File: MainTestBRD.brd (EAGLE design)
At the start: 64.4 x 62.3 mm, 27 parts, among them IC1 LM3940IMP-3.3, U1 ATMEGA128-SMD

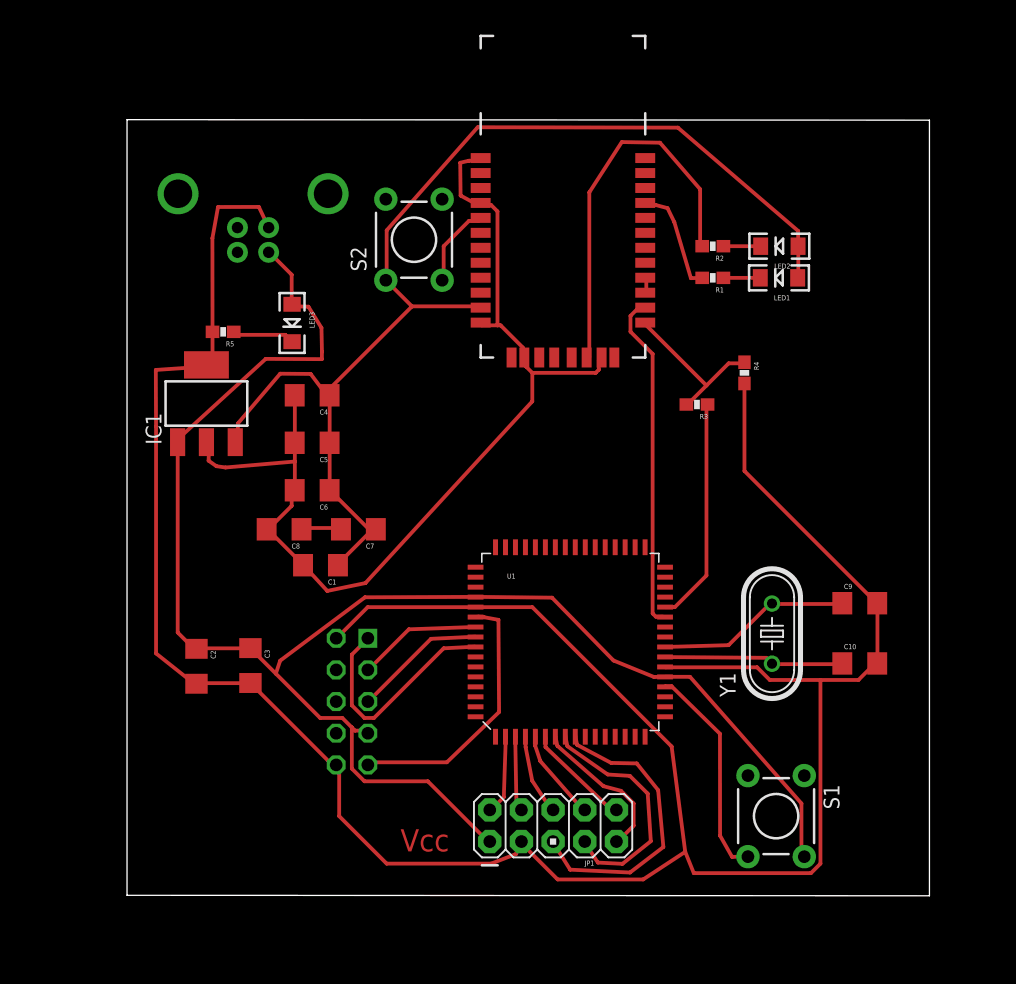
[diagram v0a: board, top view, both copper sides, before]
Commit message: __
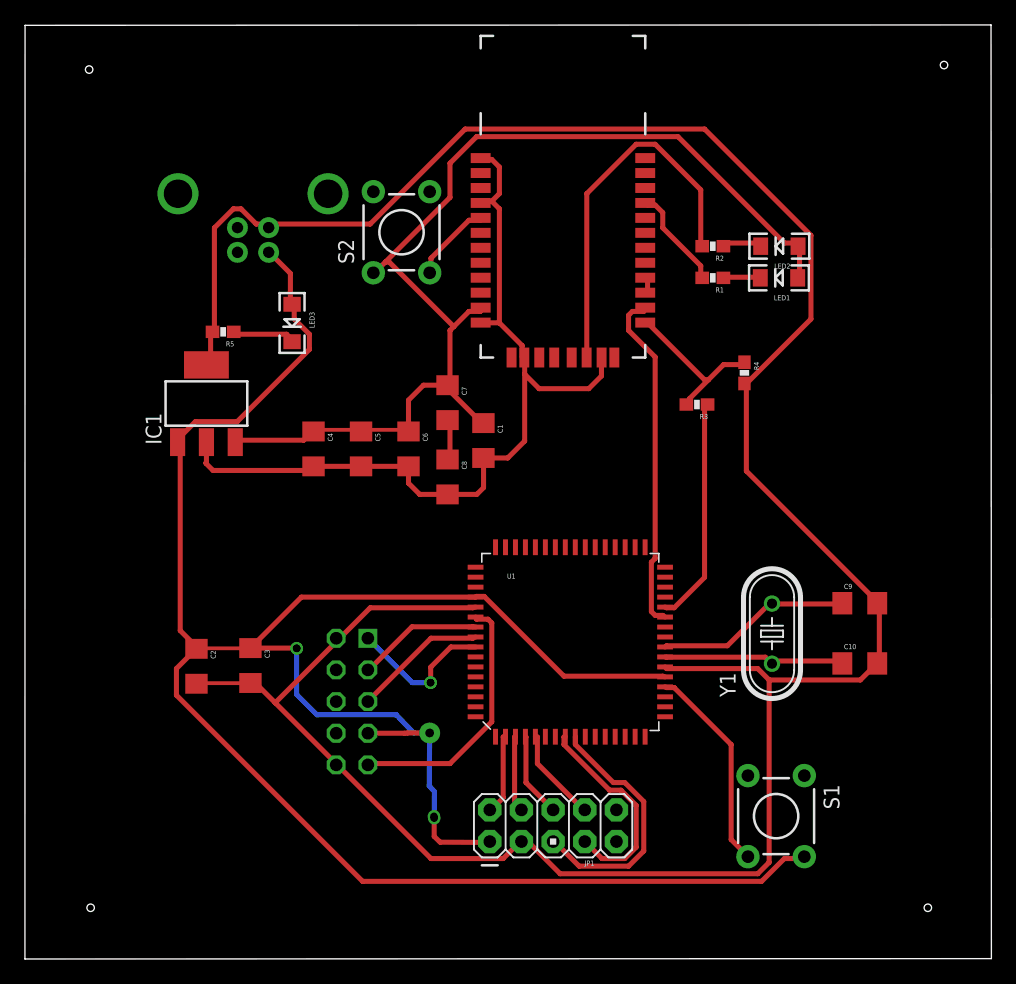
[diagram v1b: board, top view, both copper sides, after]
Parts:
- moved C1 16.5 mm to (28.6, 54.3), turned to 270 degrees
- moved C8 13.8 mm to (25.7, 51.3), turned to 270 degrees
- moved C7 12.4 mm to (25.7, 57.3), turned to 270 degrees
- moved C6 8.41 mm to (22.6, 53.6), turned to 270 degrees
- moved C4 4.30 mm to (15.0, 53.6), turned to 270 degrees
- moved C5 3.95 mm to (18.8, 53.6), turned to 270 degrees
- moved S2 1.17 mm to (22.0, 71.0)
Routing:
- net VCC: track 131.9 -> 181.9 mm, vias 0 -> 3
- net AGND: track 82.8 -> 68.7 mm
- net N$15: track 12.3 -> 0.00 mm
- net N$10: track 8.78 -> 0.00 mm
- net VDD: track 94.7 -> 87.2 mm
- net N$6: track 18.6 -> 12.0 mm, vias 0 -> 1
- net N$17: track 24.0 -> 20.5 mm
- net N$16: track 19.3 -> 16.9 mm
- net GND: track 212.6 -> 214.6 mm
- net LED2: track 31.0 -> 30.0 mm
- net N$19: track 21.5 -> 20.8 mm
- net RESET: track 17.4 -> 16.8 mm
- net BT_TX: track 27.2 -> 27.7 mm
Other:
- board size 64.4 x 62.3 mm -> 77.5 x 74.9 mm
- board text removed: "Vcc"
